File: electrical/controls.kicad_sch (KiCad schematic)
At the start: 10 parts, among them IC2 ADXL345BCCZ

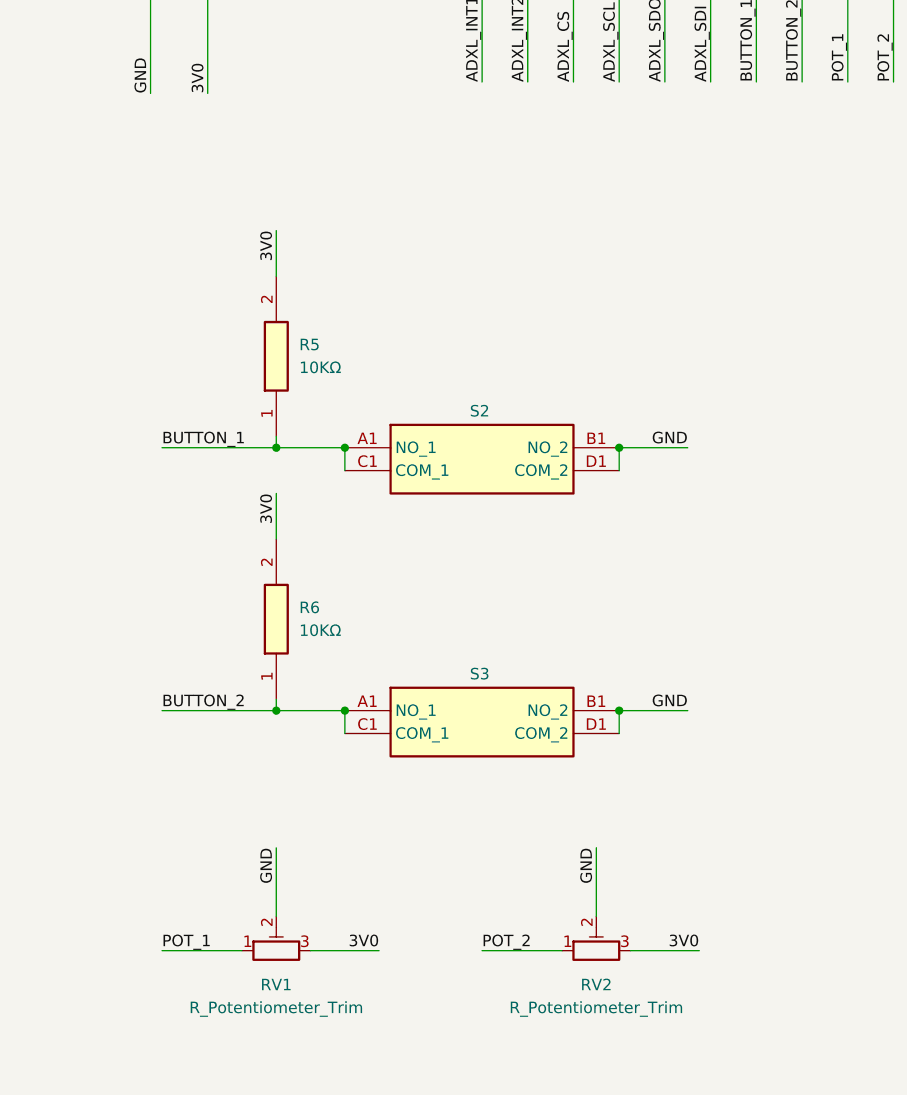
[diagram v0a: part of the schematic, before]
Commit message: not in working state yet.
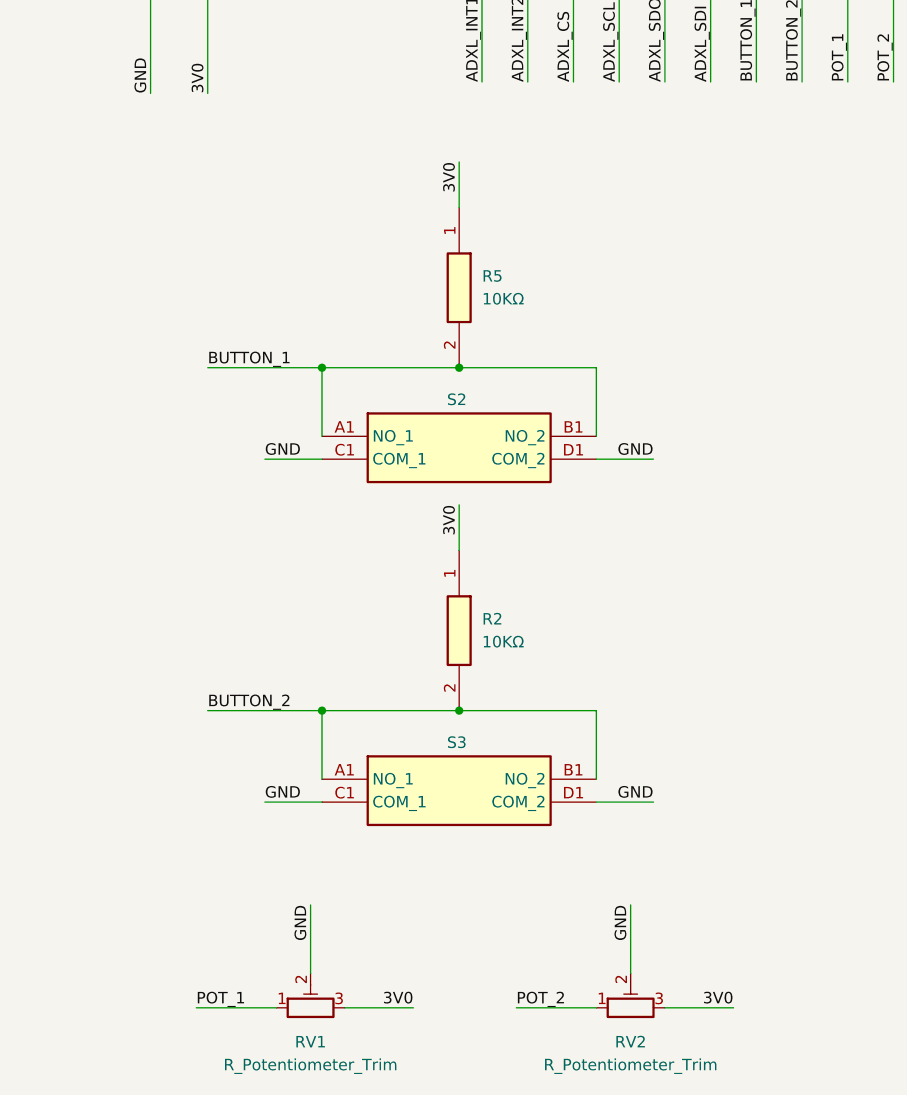
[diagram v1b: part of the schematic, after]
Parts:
- removed R6: 10KΩ, SamacSys_Parts:RESC1608X58N, symbol SamacSys_Parts:RA73F1J10KBTDF
- added R2: 10KΩ, SamacSys_Parts:RESC1608X58N, symbol SamacSys_Parts:RA73F1J10KBTDF
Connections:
- net 3V0: now also R5.1, R2.1; no longer R5.2
- net BUTTON_1: now also R5.2, S2.B1 (NO_2); no longer R5.1, S2.C1 (COM_1)
- net BUTTON_2: now also S3.B1 (NO_2), R2.2; no longer S3.C1 (COM_1)
- net GND: now also S2.C1 (COM_1), S3.C1 (COM_1); no longer S2.B1 (NO_2), S3.B1 (NO_2)
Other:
- moved on the sheet: R5, RV1, RV2, S2

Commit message: #17 Making layout. Errors rpesent.
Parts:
- IC2: footprint LGA14R80P3X6_300X500X100 -> SamacSys_Parts:LGA14R80P3X6_300X500X100
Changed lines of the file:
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@@
 		(company "AlumaPower")
+	)
+	(bus_alias "CONTROLS"
+		(members "ADXL_INT1" "ADXL_INT2" "ADXL_CS" "ADXL_SCL" "ADXL_SDO" "ADXL_SDI"
+			"BUTTON_1" "BUTTON_2" "POT_1" "POT_2"
+		)
 	)
 	(junction
@@
 			)
 		)
-		(property "Footprint" "LGA14R80P3X6_300X500X100"
+		(property "Footprint" "SamacSys_Parts:LGA14R80P3X6_300X500X100"
 			(at 250.19 186.36 0)
 			(effects
